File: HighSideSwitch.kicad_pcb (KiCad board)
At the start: 2 copper layers, 22 x 15.1 mm, 24 parts, among them J1 Conn_02x02, Q1 CSD18540Q5B, Q2 CSD18540Q5B, Q3 8050, U1 LM5060, U2 LM5050-1

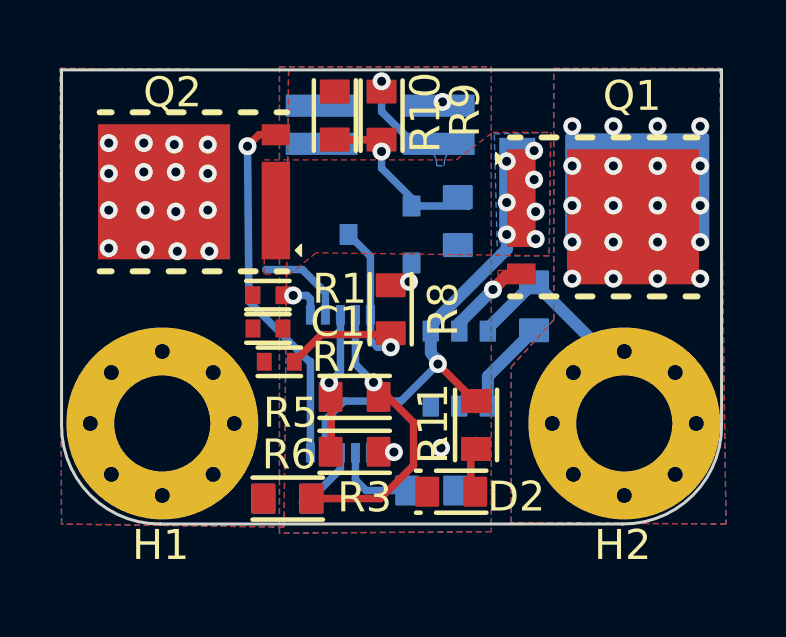
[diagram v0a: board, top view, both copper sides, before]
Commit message: small change
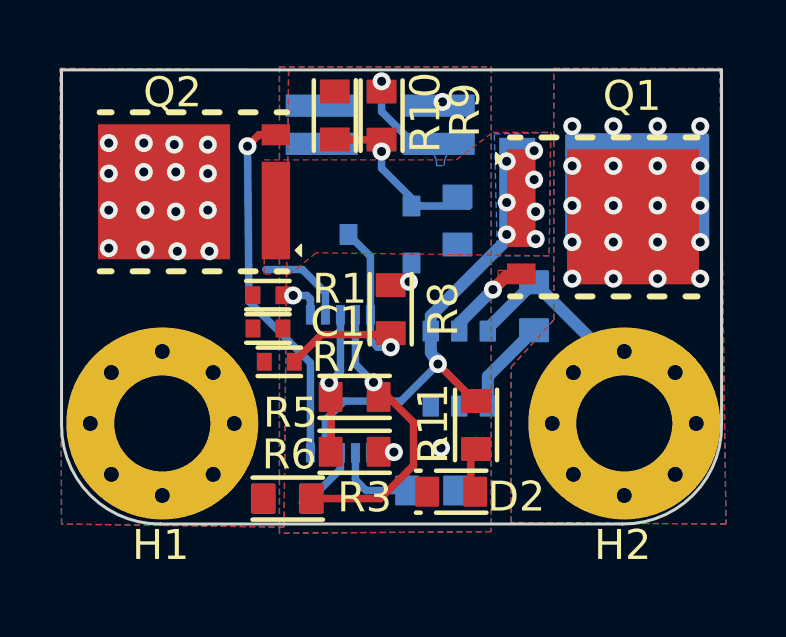
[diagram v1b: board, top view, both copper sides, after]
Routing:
- net /NMOS_OUT: track 9.46 -> 7.76 mm
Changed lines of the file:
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@@
   )
   (footprint "GENERAL_RCL_SMD:C0603(1608M)" (layer "B.Cu")
-    (at 189.3788 84.5928 90)
+    (at 189.3688 84.5728 90)
     (property "Sheetfile" "HighSideSwitch.kicad_sch")
     (property "Sheetname" "")
@@
   (segment (start 190.3776 88.2596) (end 190.3776 88.174) (width 0.4) (layer "B.Cu") (net 2))
   (segment (start 194.8744 90.146825) (end 194.8744 91.3912) (width 0.4) (layer "B.Cu") (net 2))
-  (segment (start 194.927344 89.641344) (end 194.927344 91.338256) (width 0.4) (layer "B.Cu") (net 2))
   (via (at 179.9788 82.9564) (size 0.6) (drill 0.3) (layers "F.Cu" "B.Cu") (free) (net 3))
   (via (at 178.9628 85.5472) (size 0.6) (drill 0.3) (layers "F.Cu" "B.Cu") (free) (net 3))
@@
   (segment (start 184.9652 87.8176) (end 184.9652 86.9776) (width 0.25) (layer "B.Cu") (net 3))
   (via (at 186.8388 79.9328) (size 0.6) (drill 0.3) (layers "F.Cu" "B.Cu") (free) (net 4))
-  (segment (start 186.8368 80.9414) (end 186.8368 80.4164) (width 0.25) (layer "B.Cu") (net 4))
+  (segment (start 186.8368 79.9348) (end 186.8388 79.9328) (width 0.25) (layer "B.Cu") (net 4))
+  (segment (start 186.8368 80.9414) (end 186.8368 79.9348) (width 0.25) (layer "B.Cu") (net 4))
   (segment (start 187.9116 82.0162) (end 186.8368 80.9414) (width 0.25) (layer "B.Cu") (net 4))
   (segment (start 186.720289 88.377089) (end 184.834511 88.377089) (width 0.25) (layer "F.Cu") (net 5))
@@
   (segment (start 188.096 84.0892) (end 189.7196 84.0892) (width 0.25) (layer "B.Cu") (net 10))
   (segment (start 189.7196 84.0892) (end 189.7324 84.102) (width 0.25) (layer "B.Cu") (net 10))
-  (segment (start 186.8368 81.8388) (end 186.8368 82.83) (width 0.25) (layer "B.Cu") (net 10))
+  (segment (start 186.8368 82.83) (end 186.8368 82.2728) (width 0.25) (layer "B.Cu") (net 10))
   (segment (start 186.8368 82.83) (end 188.096 84.0892) (width 0.25) (layer "B.Cu") (net 10))
   (segment (start 189.9864 90.8792) (end 189.9864 90.6272) (width 0.25) (layer "F.Cu") (net 11))
@@
   (segment (start 188.7164 89.3572) (end 188.7164 89.2048) (width 0.4) (layer "B.Cu") (net 11))
   (segment (start 187.4888 90.5928) (end 188.7164 89.3652) (width 0.25) (layer "B.Cu") (net 11))
-  (segment (start 191.008 85.0392) (end 191.008 85.531526) (width 0.4) (layer "B.Cu") (net 11))
-  (segment (start 188.4776 88.061926) (end 188.4776 88.2596) (width 0.4) (layer "B.Cu") (net 11))
+  (segment (start 191.008 85.2236) (end 188.4776 87.754) (width 0.4) (layer "B.Cu") (net 11))
+  (segment (start 188.4776 87.754) (end 188.4776 88.2596) (width 0.4) (layer "B.Cu") (net 11))
   (segment (start 188.7164 89.3572) (end 188.4776 88.966) (width 0.4) (layer "B.Cu") (net 11))
   (segment (start 188.4776 88.966) (end 188.4776 88.2596) (width 0.4) (layer "B.Cu") (net 11))
+  (segment (start 191.008 85.0392) (end 191.008 85.2236) (width 0.4) (layer "B.Cu") (net 11))
   (segment (start 184.9652 92.2176) (end 184.9652 91.218578) (width 0.25) (layer "B.Cu") (net 11))
   (segment (start 184.9652 91.218578) (end 185.590978 90.5928) (width 0.25) (layer "B.Cu") (net 11))
-  (segment (start 191.008 85.531526) (end 188.4776 88.061926) (width 0.4) (layer "B.Cu") (net 11))
   (segment (start 185.590978 90.5928) (end 187.4888 90.5928) (width 0.25) (layer "B.Cu") (net 11))
   (segment (start 189.8087 92.0769) (end 189.9864 91.8992) (width 0.25) (layer "F.Cu") (net 12))
@@
   (segment (start 182.753595 81.7118) (end 182.368496 82.096899) (width 0.25) (layer "F.Cu") (net 14))
   (via (at 182.368496 82.096899) (size 0.6) (drill 0.3) (layers "F.Cu" "B.Cu") (free) (net 14))
+  (segment (start 184.4652 92.3176) (end 184.4652 89.316622) (width 0.25) (layer "B.Cu") (net 14))
   (segment (start 182.4172 87.268622) (end 182.368496 82.096899) (width 0.25) (layer "B.Cu") (net 14))
-  (segment (start 184.4652 89.2716) (end 184.420178 89.2716) (width 0.25) (layer "B.Cu") (net 14))
   (segment (start 182.368496 82.096899) (end 182.4172 82.042) (width 0.25) (layer "B.Cu") (net 14))
-  (segment (start 184.4652 92.2176) (end 184.4652 89.2716) (width 0.25) (layer "B.Cu") (net 14))
-  (segment (start 184.420178 89.2716) (end 182.4172 87.268622) (width 0.25) (layer "B.Cu") (net 14))
+  (segment (start 184.4652 89.316622) (end 182.4172 87.268622) (width 0.25) (layer "B.Cu") (net 14))
   (segment (start 186.5688 89.9683) (end 187.9036 91.3031) (width 0.25) (layer "F.Cu") (net 15))
   (segment (start 186.793291 93.8428) (end 184.5088 93.8428) (width 0.25) (layer "F.Cu") (net 15))

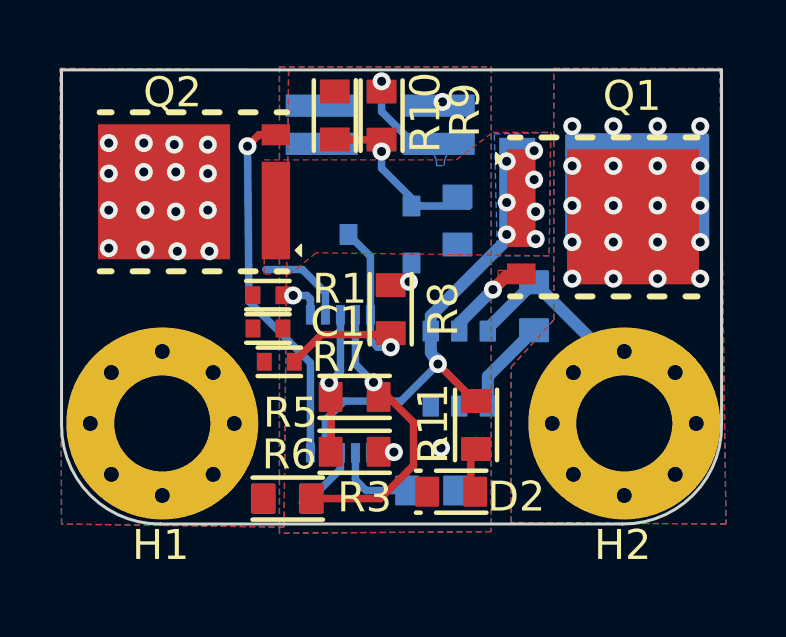
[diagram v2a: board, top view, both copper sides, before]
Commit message: another right version
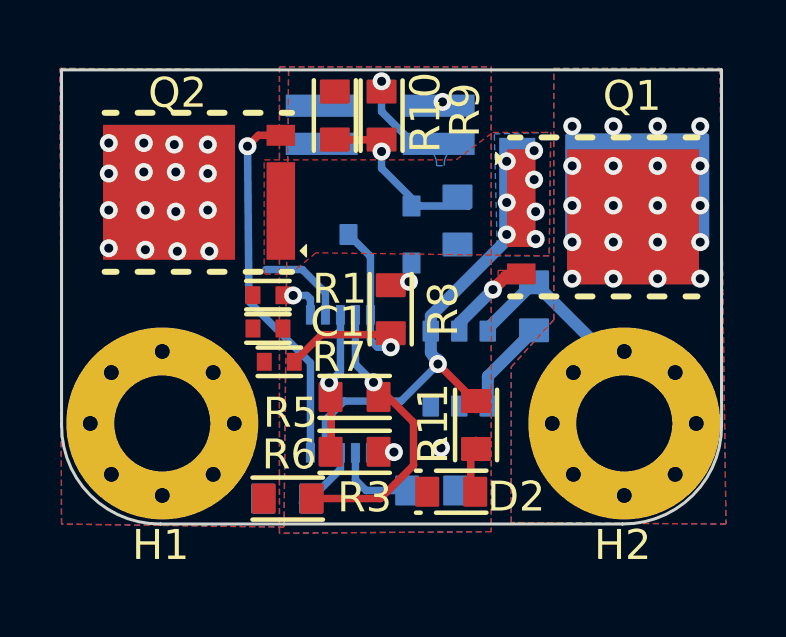
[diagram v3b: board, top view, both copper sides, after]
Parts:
- moved Q2 0.17 mm to (180.8, 83.6)
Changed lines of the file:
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@@
   )
   (footprint "POWER_TRANSISTOR_SMD:SON-6050-FET" (layer "F.Cu")
-    (at 180.5884 83.6168 90)
+    (at 180.7538 83.6328 90)
     (descr "Footprint for single MOSFET")
     (property "Sheetfile" "HighSideSwitch.kicad_sch")
@@
   (segment (start 189.4276 87.995119) (end 189.4276 88.3721) (width 0.4) (layer "B.Cu") (net 13))
   (segment (start 190.548629 86.87409) (end 189.4276 87.995119) (width 0.4) (layer "B.Cu") (net 13))
-  (segment (start 183.4884 81.7118) (end 182.753595 81.7118) (width 0.25) (layer "F.Cu") (net 14))
-  (segment (start 182.753595 81.7118) (end 182.368496 82.096899) (width 0.25) (layer "F.Cu") (net 14))
+  (segment (start 182.732595 81.7328) (end 182.368496 82.096899) (width 0.25) (layer "F.Cu") (net 14))
+  (segment (start 183.4788 81.7328) (end 182.732595 81.7328) (width 0.25) (layer "F.Cu") (net 14))
   (via (at 182.368496 82.096899) (size 0.6) (drill 0.3) (layers "F.Cu" "B.Cu") (free) (net 14))
   (segment (start 184.4652 92.3176) (end 184.4652 89.316622) (width 0.25) (layer "B.Cu") (net 14))

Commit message: another right version
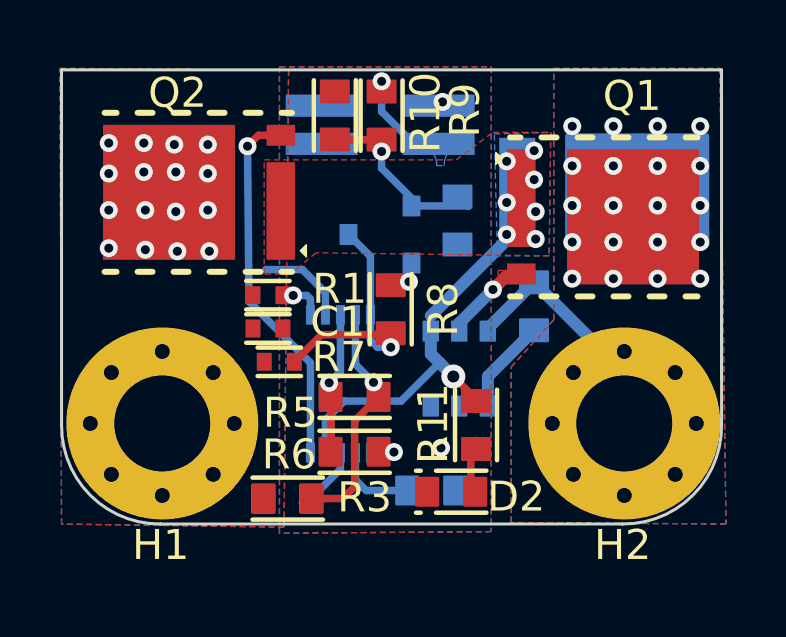
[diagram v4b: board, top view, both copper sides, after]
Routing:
- net Net-(R3-Pad1): track 9.57 -> 7.32 mm
- net Net-(Q2-PadS): track 13.2 -> 12.6 mm
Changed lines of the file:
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@@
   (segment (start 186.8368 82.83) (end 186.8368 82.2728) (width 0.25) (layer "B.Cu") (net 10))
   (segment (start 186.8368 82.83) (end 188.096 84.0892) (width 0.25) (layer "B.Cu") (net 10))
+  (segment (start 189.9864 90.5892) (end 189.9864 90.5304) (width 0.25) (layer "F.Cu") (net 11))
   (segment (start 189.9864 90.8792) (end 189.9864 90.6272) (width 0.25) (layer "F.Cu") (net 11))
-  (segment (start 189.9864 90.6272) (end 188.7164 89.3572) (width 0.25) (layer "F.Cu") (net 11))
+  (segment (start 189.9864 90.5304) (end 189.2288 89.7728) (width 0.25) (layer "F.Cu") (net 11))
   (via (at 191.9732 85.1916) (size 0.6) (drill 0.3) (layers "F.Cu" "B.Cu") (free) (net 11))
   (via (at 191.9732 84.2772) (size 0.6) (drill 0.3) (layers "F.Cu" "B.Cu") (free) (net 11))
-  (via (at 188.7164 89.3572) (size 0.6) (drill 0.3) (layers "F.Cu" "B.Cu") (free) (net 11))
   (via (at 191.008 82.6008) (size 0.6) (drill 0.3) (layers "F.Cu" "B.Cu") (free) (net 11))
   (via (at 191.9224 82.2452) (size 0.6) (drill 0.3) (layers "F.Cu" "B.Cu") (free) (net 11))
   (via (at 191.008 85.0392) (size 0.6) (drill 0.3) (layers "F.Cu" "B.Cu") (free) (net 11))
   (via (at 191.008 83.9724) (size 0.6) (drill 0.3) (layers "F.Cu" "B.Cu") (free) (net 11))
+  (via (at 189.2288 89.7728) (size 0.8) (drill 0.4) (layers "F.Cu" "B.Cu") (net 11))
   (via (at 191.9224 83.2104) (size 0.6) (drill 0.3) (layers "F.Cu" "B.Cu") (free) (net 11))
-  (segment (start 188.7164 89.3652) (end 188.7164 89.3572) (width 0.25) (layer "B.Cu") (net 11))
-  (segment (start 188.7164 89.3572) (end 188.7164 89.2048) (width 0.4) (layer "B.Cu") (net 11))
-  (segment (start 187.4888 90.5928) (end 188.7164 89.3652) (width 0.25) (layer "B.Cu") (net 11))
   (segment (start 191.008 85.2236) (end 188.4776 87.754) (width 0.4) (layer "B.Cu") (net 11))
-  (segment (start 188.4776 87.754) (end 188.4776 88.2596) (width 0.4) (layer "B.Cu") (net 11))
-  (segment (start 188.7164 89.3572) (end 188.4776 88.966) (width 0.4) (layer "B.Cu") (net 11))
-  (segment (start 188.4776 88.966) (end 188.4776 88.2596) (width 0.4) (layer "B.Cu") (net 11))
+  (segment (start 187.4888 90.5928) (end 188.7638 89.3178) (width 0.25) (layer "B.Cu") (net 11))
+  (segment (start 188.4776 89.0216) (end 188.4776 88.2596) (width 0.4) (layer "B.Cu") (net 11))
+  (segment (start 188.7638 89.3178) (end 188.7738 89.3178) (width 0.25) (layer "B.Cu") (net 11))
+  (segment (start 189.2288 89.7728) (end 188.7738 89.3178) (width 0.4) (layer "B.Cu") (net 11))
   (segment (start 191.008 85.0392) (end 191.008 85.2236) (width 0.4) (layer "B.Cu") (net 11))
+  (segment (start 188.7738 89.3178) (end 188.4776 89.0216) (width 0.4) (layer "B.Cu") (net 11))
   (segment (start 184.9652 92.2176) (end 184.9652 91.218578) (width 0.25) (layer "B.Cu") (net 11))
   (segment (start 184.9652 91.218578) (end 185.590978 90.5928) (width 0.25) (layer "B.Cu") (net 11))
@@
   (segment (start 182.368496 82.096899) (end 182.4172 82.042) (width 0.25) (layer "B.Cu") (net 14))
   (segment (start 184.4652 89.316622) (end 182.4172 87.268622) (width 0.25) (layer "B.Cu") (net 14))
-  (segment (start 186.5688 89.9683) (end 187.9036 91.3031) (width 0.25) (layer "F.Cu") (net 15))
-  (segment (start 186.793291 93.8428) (end 184.5088 93.8428) (width 0.25) (layer "F.Cu") (net 15))
-  (segment (start 187.9036 92.732491) (end 186.793291 93.8428) (width 0.25) (layer "F.Cu") (net 15))
-  (segment (start 187.9036 91.3031) (end 187.9036 92.732491) (width 0.25) (layer "F.Cu") (net 15))
+  (segment (start 185.9388 93.4428) (end 185.5388 93.8428) (width 0.25) (layer "F.Cu") (net 15))
+  (segment (start 185.5388 93.8428) (end 184.5088 93.8428) (width 0.25) (layer "F.Cu") (net 15))
+  (segment (start 185.9388 91.2528) (end 185.9388 93.4428) (width 0.25) (layer "F.Cu") (net 15))
+  (segment (start 186.7388 90.4528) (end 185.9388 91.2528) (width 0.25) (layer "F.Cu") (net 15))
   (via (at 186.5688 89.9683) (size 0.6) (drill 0.3) (layers "F.Cu" "B.Cu") (free) (net 15))
   (segment (start 186.5688 89.9683) (end 185.9652 89.3647) (width 0.25) (layer "B.Cu") (net 15))

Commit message: final
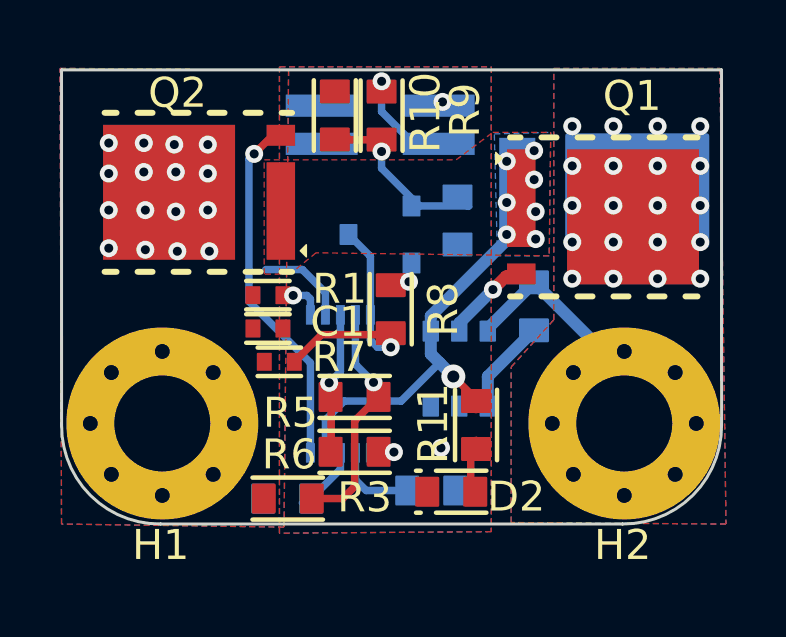
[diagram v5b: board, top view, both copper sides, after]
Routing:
- net Net-(Q2-PadS): track 12.6 -> 13.1 mm
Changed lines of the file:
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@@
   (via (at 189.2288 89.7728) (size 0.8) (drill 0.4) (layers "F.Cu" "B.Cu") (net 11))
   (via (at 191.9224 83.2104) (size 0.6) (drill 0.3) (layers "F.Cu" "B.Cu") (free) (net 11))
+  (segment (start 188.4776 87.754) (end 188.4776 88.2596) (width 0.4) (layer "B.Cu") (net 11))
   (segment (start 191.008 85.2236) (end 188.4776 87.754) (width 0.4) (layer "B.Cu") (net 11))
   (segment (start 187.4888 90.5928) (end 188.7638 89.3178) (width 0.25) (layer "B.Cu") (net 11))
@@
   (segment (start 189.4276 87.995119) (end 189.4276 88.3721) (width 0.4) (layer "B.Cu") (net 13))
   (segment (start 190.548629 86.87409) (end 189.4276 87.995119) (width 0.4) (layer "B.Cu") (net 13))
-  (segment (start 182.732595 81.7328) (end 182.368496 82.096899) (width 0.25) (layer "F.Cu") (net 14))
-  (segment (start 183.4788 81.7328) (end 182.732595 81.7328) (width 0.25) (layer "F.Cu") (net 14))
-  (via (at 182.368496 82.096899) (size 0.6) (drill 0.3) (layers "F.Cu" "B.Cu") (free) (net 14))
-  (segment (start 184.4652 92.3176) (end 184.4652 89.316622) (width 0.25) (layer "B.Cu") (net 14))
-  (segment (start 182.4172 87.268622) (end 182.368496 82.096899) (width 0.25) (layer "B.Cu") (net 14))
-  (segment (start 182.368496 82.096899) (end 182.4172 82.042) (width 0.25) (layer "B.Cu") (net 14))
-  (segment (start 184.4652 89.316622) (end 182.4172 87.268622) (width 0.25) (layer "B.Cu") (net 14))
+  (segment (start 182.590358 82.3525) (end 183.210058 81.7328) (width 0.25) (layer "F.Cu") (net 14))
+  (segment (start 183.210058 81.7328) (end 183.4788 81.7328) (width 0.25) (layer "F.Cu") (net 14))
+  (via (at 182.590358 82.3525) (size 0.6) (drill 0.3) (layers "F.Cu" "B.Cu") (free) (net 14))
+  (segment (start 182.590358 82.3525) (end 182.590358 82.215158) (width 0.25) (layer "B.Cu") (net 14))
+  (segment (start 182.4172 87.268622) (end 184.4652 89.316622) (width 0.25) (layer "B.Cu") (net 14))
+  (segment (start 184.4652 89.316622) (end 184.4652 92.3176) (width 0.25) (layer "B.Cu") (net 14))
+  (segment (start 182.590358 82.3525) (end 182.4172 82.525658) (width 0.25) (layer "B.Cu") (net 14))
+  (segment (start 182.4172 82.525658) (end 182.4172 87.268622) (width 0.25) (layer "B.Cu") (net 14))
   (segment (start 185.9388 93.4428) (end 185.5388 93.8428) (width 0.25) (layer "F.Cu") (net 15))
   (segment (start 185.5388 93.8428) (end 184.5088 93.8428) (width 0.25) (layer "F.Cu") (net 15))
@@
     )
   )
-  (zone (net 0) (net_name "") (layer "F.Cu") (hatch edge 0.508)
-    (priority 16962)
-    (connect_pads yes (clearance 0))
-    (min_thickness 0.0254) (filled_areas_thickness no)
-    (fill yes (thermal_gap 0.508) (thermal_bridge_width 0.508) (island_removal_mode 1) (island_area_min 0))
-    (polygon
-      (pts
-        (xy 190.7204 86.6362)
-        (xy 190.775143 86.635776)
-        (xy 190.825093 86.634805)
-        (xy 190.870661 86.633735)
-        (xy 190.912257 86.633016)
-        (xy 190.950291 86.633096)
-        (xy 190.985176 86.634424)
-        (xy 191.017321 86.637449)
-        (xy 191.047138 86.642621)
-        (xy 191.075036 86.650388)
-        (xy 191.101428 86.6612)
-        (xy 191.3354 86.4362)
-        (xy 191.101428 86.2112)
-        (xy 191.075036 86.222011)
-        (xy 191.047138 86.229778)
-        (xy 191.017321 86.23495)
-        (xy 190.985176 86.237975)
-        (xy 190.950291 86.239303)
-        (xy 190.912257 86.239383)
-        (xy 190.870661 86.238664)
-        (xy 190.825093 86.237594)
-        (xy 190.775143 86.236623)
-        (xy 190.7204 86.2362)
-      )
-    )
-  )
   (zone (net 11) (net_name "Net-(Q2-PadS)") (layer "B.Cu") (hatch edge 0.508)
     (priority 3)
@@
       )
     )
-  )
-  (zone (net 4) (net_name "/~{EN}") (layer "B.Cu") (hatch edge 0.508)
-    (priority 16962)
-    (connect_pads yes (clearance 0))
-    (min_thickness 0.0254) (filled_areas_thickness no)
-    (fill yes (thermal_gap 0.508) (thermal_bridge_width 0.508) (island_removal_mode 1) (island_area_min 0))
-    (polygon
-      (pts
-        (xy 188.9244 82.7462)
-        (xy 188.927198 82.662946)
-        (xy 188.935275 82.592994)
-        (xy 188.94815 82.533554)
-        (xy 188.965346 82.481837)
-        (xy 188.986382 82.435052)
-        (xy 189.010779 82.39041)
-        (xy 189.038058 82.345122)
-        (xy 189.067741 82.296397)
-        (xy 189.099348 82.241446)
-        (xy 189.1324 82.177479)
-        (xy 188.7994 81.8312)
-        (xy 188.4664 82.177479)
-        (xy 188.499451 82.241446)
-        (xy 188.531058 82.296397)
-        (xy 188.560741 82.345122)
-        (xy 188.58802 82.39041)
-        (xy 188.612417 82.435052)
-        (xy 188.633453 82.481837)
-        (xy 188.650649 82.533554)
-        (xy 188.663524 82.592994)
-        (xy 188.671601 82.662946)
-        (xy 188.6744 82.7462)
-      )
-    )

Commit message: final
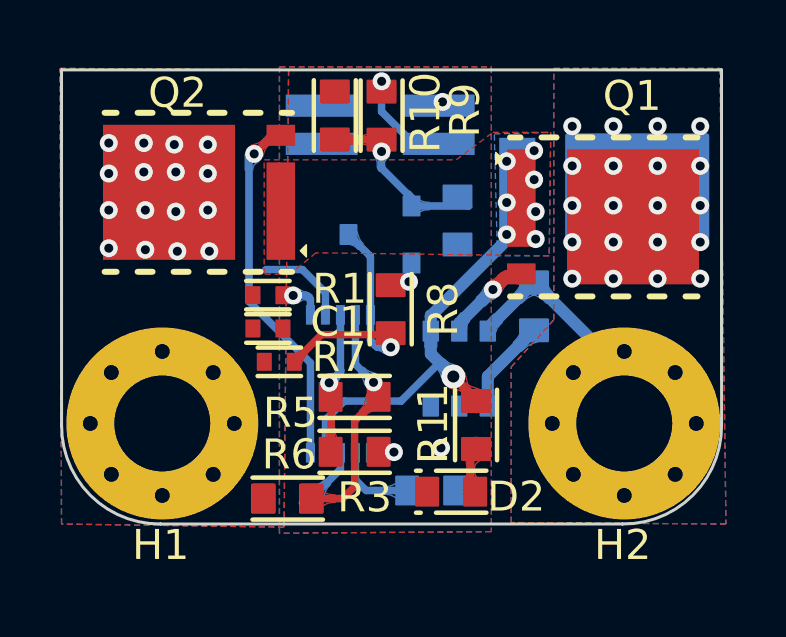
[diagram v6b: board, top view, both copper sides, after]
